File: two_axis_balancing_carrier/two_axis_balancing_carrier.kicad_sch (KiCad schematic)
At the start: 8 parts, among them J1 Conn_01x03, J5 Conn_02x05, U1 NUCLEO-G474RE, U2 MIC5219-3.3YM5, U3 ICM-42688-P, U4 SN65HVD230

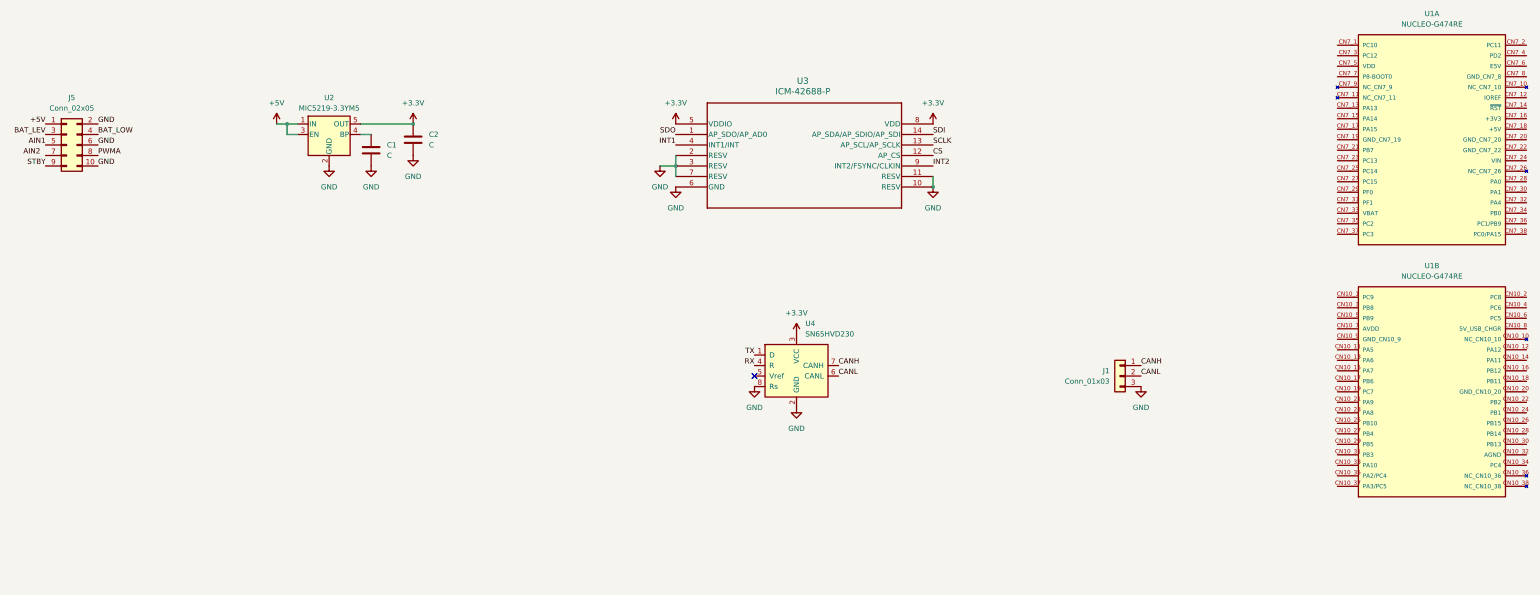
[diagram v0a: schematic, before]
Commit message: Finished topology
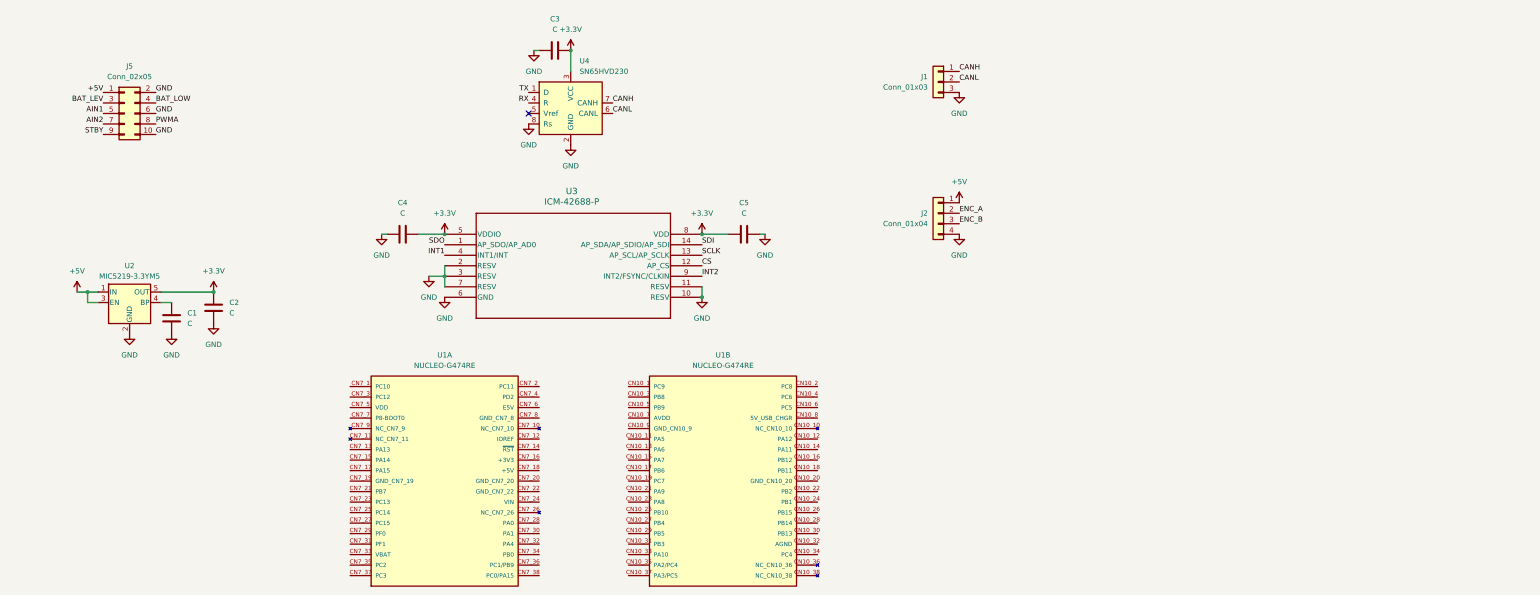
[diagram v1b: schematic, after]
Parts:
- added C3, C4, C5: C, symbol Device:C
- added J2: Conn_01x04, symbol Connector_Generic:Conn_01x04
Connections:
- net +3.3V: now also C3.1, C4.2, C5.2
- net +5V: now also J2.1 (Pin_1)
- net AIN2: now also J5.7 (Pin_7)
- net GND: now also C3.2, C4.1, C5.1, J2.4 (Pin_4)
- new net ENC_A: J2.2 (Pin_2)
- new net ENC_B: J2.3 (Pin_3)
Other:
- moved on the sheet: C1, C2, J1, J5, U1A, U1B, U2, U3, U4
